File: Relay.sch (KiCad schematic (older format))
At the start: 0 parts

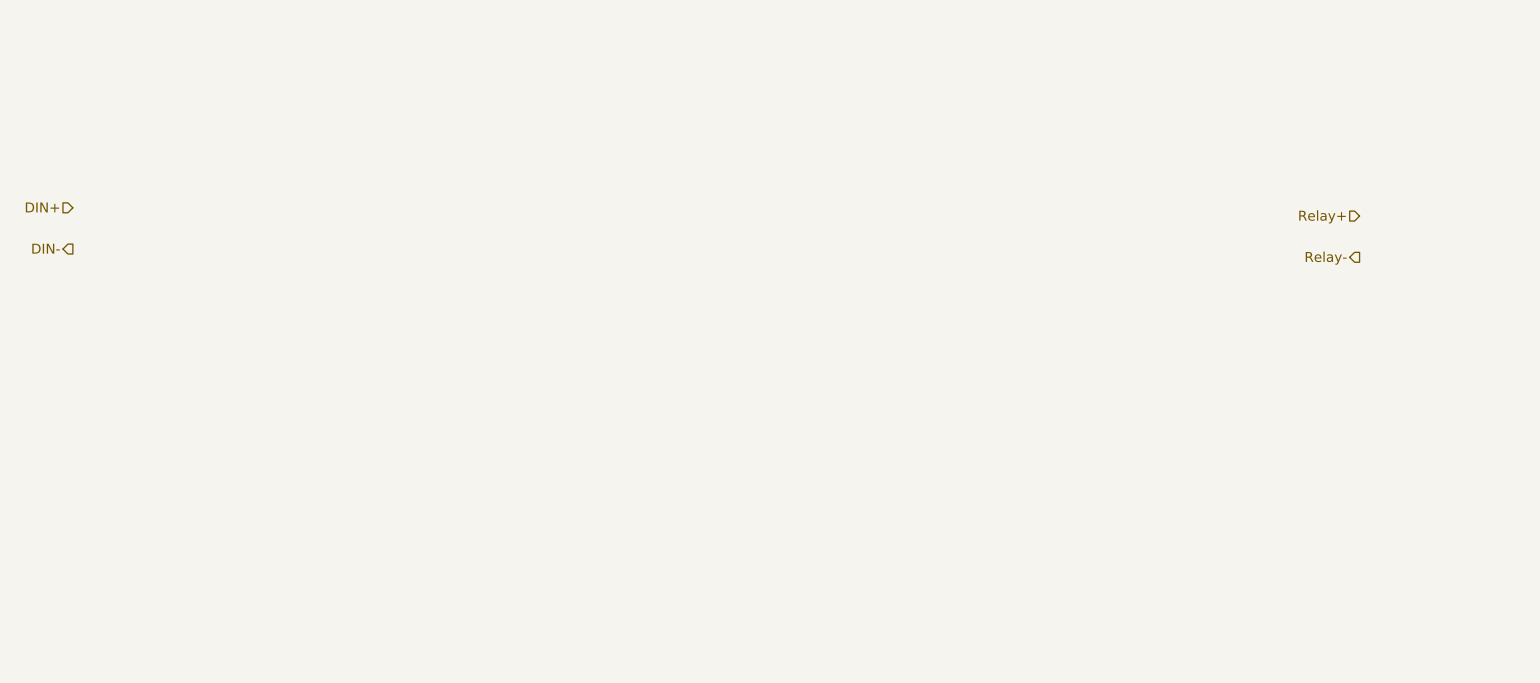
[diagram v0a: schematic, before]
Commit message: Module 3, Unit 5: Understanding The Relay Module
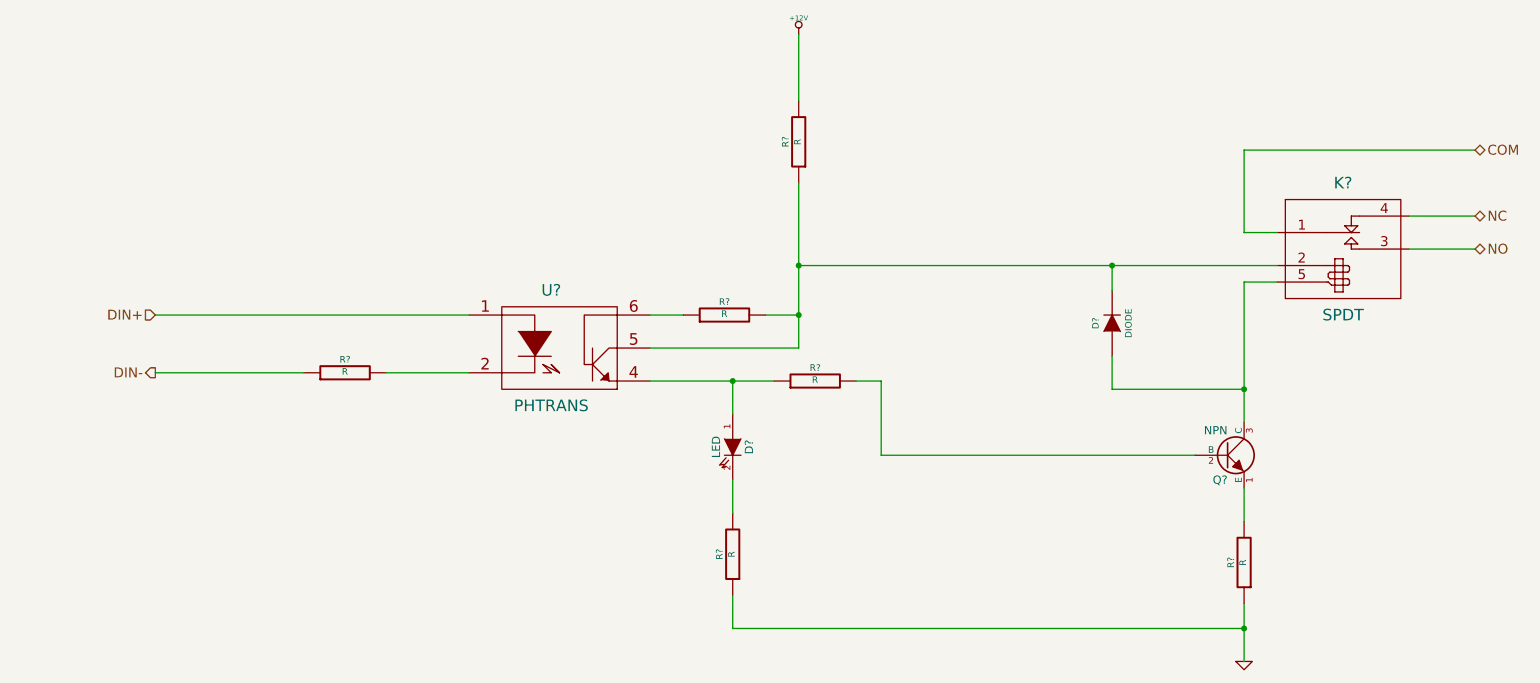
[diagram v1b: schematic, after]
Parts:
- added D?: LED, symbol LED
- added D?: DIODE, symbol DIODE
- added K?: SPDT, symbol SPDT
- added Q?: NPN, symbol NPN
- added R? (x6): R, symbol R
- added U?: PHTRANS, symbol PHTRANS
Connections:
- net DIN+: now also U?.1
- net DIN-: now also R?.1
- new net: R?.2, U?.2
- new net: D?.1 (A), R?.1, U?.4
- new net: D?.2 (K), K?.2 (COIL+), R?.1, R?.2, U?.5
- new net: R?.1, U?.6
- new net: Q?.2 (B), R?.2
- new net: Q?.1 (E), R?.2
- new net: D?.1 (A), K?.5 (COIL-), Q?.3 (C)
- new net: D?.2 (K), R?.2
- new net +12V: R?.2
- new net COM: K?.1 (COM)
- new net GND: R?.1, R?.1
- new net NC: K?.4 (NC)
- new net NO: K?.3 (NO)
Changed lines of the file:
@@
 LIBS:contrib
 LIBS:valves
+LIBS:BenchBudEE
 LIBS:BenchBudEE-cache
 EELAYER 24 0
@@
 Comment4 ""
 $EndDescr
-Text HLabel 2000 2550 0    60   Input ~ 0
+Text HLabel 2500 3200 0    60   Input ~ 0
 DIN+
-Text HLabel 2000 2800 0    60   Output ~ 0
+Text HLabel 2500 3550 0    60   Output ~ 0
 DIN-
-Text HLabel 9800 2600 0    60   Input ~ 0
-Relay+
-Text HLabel 9800 2850 0    60   Output ~ 0
-Relay-
+Text HLabel 10500 2600 2    60   BiDi ~ 0
+NC
+Text HLabel 10500 2800 2    60   BiDi ~ 0
+NO
+$Comp
+L PHTRANS U?
+U 1 1 53012FD3
+P 4950 3400
+F 0 "U?" H 4900 3750 70  0000 C CNN
+F 1 "PHTRANS" H 4900 3050 70  0000 C CNN
+F 2 "" H 4950 3400 60  0000 C CNN
+F 3 "" H 4950 3400 60  0000 C CNN
+	1    4950 3400
+	1    0    0    -1
+$EndComp
+$Comp
+L R R?
+U 1 1 53012FF1
+P 6500 3600
+F 0 "R?" V 6580 3600 40  0000 C CNN
+F 1 "R" V 6507 3601 40  0000 C CNN
+F 2 "" V 6430 3600 30  0000 C CNN
+F 3 "" H 6500 3600 30  0000 C CNN
+	1    6500 3600
+	0    -1   -1   0
+$EndComp
+$Comp
+L NPN Q?
+U 1 1 53013005
+P 9000 4050
+F 0 "Q?" H 9000 3900 50  0000 R CNN
+F 1 "NPN" H 9000 4200 50  0000 R CNN
+F 2 "" H 9000 4050 60  0000 C CNN
+F 3 "" H 9000 4050 60  0000 C CNN
+	1    9000 4050
+	1    0    0    -1
+$EndComp
+$Comp
+L LED D?
+U 1 1 53013023
+P 6000 4000
+F 0 "D?" H 6000 4100 50  0000 C CNN
+F 1 "LED" H 6000 3900 50  0000 C CNN
+F 2 "" H 6000 4000 60  0000 C CNN
+F 3 "" H 6000 4000 60  0000 C CNN
+	1    6000 4000
+	0    1    1    0
+$EndComp
+$Comp
+L SPDT K?
+U 1 1 5301353C
+P 9700 2650
+F 0 "K?" H 9700 2900 70  0000 C CNN
+F 1 "SPDT" H 9700 2100 70  0000 C CNN
+F 2 "" H 9700 2650 60  0000 C CNN
+F 3 "" H 9700 2650 60  0000 C CNN
+	1    9700 2650
+	1    0    0    -1
+$EndComp
+Text HLabel 10500 2200 2    60   BiDi ~ 0
+COM
+Wire Wire Line
+	10100 2600 10500 2600
+Wire Wire Line
+	10100 2800 10500 2800
+Wire Wire Line
+	5500 3600 6250 3600
+Wire Wire Line
+	9100 3000 9300 3000
+$Comp
+L GND #PWR?
+U 1 1 53013B82
+P 9100 5300
+F 0 "#PWR?" H 9100 5300 30  0001 C CNN
+F 1 "GND" H 9100 5230 30  0001 C CNN
+F 2 "" H 9100 5300 60  0000 C CNN
+F 3 "" H 9100 5300 60  0000 C CNN
+	1    9100 5300
+	1    0    0    -1
+$EndComp
+$Comp
+L R R?
+U 1 1 53013B9D
+P 9100 4700
+F 0 "R?" V 9180 4700 40  0000 C CNN
+F 1 "R" V 9107 4701 40  0000 C CNN
+F 2 "" V 9030 4700 30  0000 C CNN
+F 3 "" H 9100 4700 30  0000 C CNN
+	1    9100 4700
+	-1   0    0    1
+$EndComp
+Wire Wire Line
+	9100 4950 9100 5300
+$Comp
+L R R?
+U 1 1 53013BD9
+P 6000 4650
+F 0 "R?" V 6080 4650 40  0000 C CNN
+F 1 "R" V 6007 4651 40  0000 C CNN
+F 2 "" V 5930 4650 30  0000 C CNN
+F 3 "" H 6000 4650 30  0000 C CNN
+	1    6000 4650
+	-1   0    0    1
+$EndComp
+Wire Wire Line
+	6000 3800 6000 3600
+Connection ~ 6000 3600
+Wire Wire Line
+	6000 4200 6000 4400
+Wire Wire Line
+	6000 4900 6000 5100
+Wire Wire Line
+	6000 5100 9100 5100
+Connection ~ 9100 5100
+$Comp
+L R R?
+U 1 1 53013C23
+P 6400 2150
+F 0 "R?" V 6480 2150 40  0000 C CNN
+F 1 "R" V 6407 2151 40  0000 C CNN
+F 2 "" V 6330 2150 30  0000 C CNN
+F 3 "" H 6400 2150 30  0000 C CNN
+	1    6400 2150
+	-1   0    0    1
+$EndComp
+$Comp
+L +12V #PWR?
+U 1 1 53013C30
+P 6400 1500
+F 0 "#PWR?" H 6400 1450 20  0001 C CNN
+F 1 "+12V" H 6400 1600 30  0000 C CNN
+F 2 "" H 6400 1500 60  0000 C CNN
+F 3 "" H 6400 1500 60  0000 C CNN
+	1    6400 1500
+	1    0    0    -1
+$EndComp
+Wire Wire Line
+	6400 1500 6400 1900
+Wire Wire Line
+	6400 2400 6400 3400
+Wire Wire Line
+	6400 2900 9300 2900
+Wire Wire Line
+	6400 3400 5500 3400
+Connection ~ 6400 2900
+$Comp
+L R R?
+U 1 1 53013C87
+P 5950 3200
+F 0 "R?" V 6030 3200 40  0000 C CNN
+F 1 "R" V 5957 3201 40  0000 C CNN
+F 2 "" V 5880 3200 30  0000 C CNN
+F 3 "" H 5950 3200 30  0000 C CNN
+	1    5950 3200
+	0    -1   -1   0
+$EndComp
+Wire Wire Line
+	5500 3200 5700 3200
+Wire Wire Line
+	6200 3200 6400 3200
+Connection ~ 6400 3200
+$Comp
+L R R?
+U 1 1 53013CC0
+P 3650 3550
+F 0 "R?" V 3730 3550 40  0000 C CNN
+F 1 "R" V 3657 3551 40  0000 C CNN
+F 2 "" V 3580 3550 30  0000 C CNN
+F 3 "" H 3650 3550 30  0000 C CNN
+	1    3650 3550
+	0    -1   -1   0
+$EndComp
+Wire Wire Line
+	2500 3200 4400 3200
+Wire Wire Line
+	3900 3550 4400 3550
+Wire Wire Line
+	3400 3550 2500 3550
+Wire Wire Line
+	10500 2200 9100 2200
+Wire Wire Line
+	9100 2200 9100 2700
+Wire Wire Line
+	9100 2700 9300 2700
+$Comp
+L DIODE D?
+U 1 1 53013E0F
+P 8300 3250
+F 0 "D?" H 8300 3350 40  0000 C CNN
+F 1 "DIODE" H 8300 3150 40  0000 C CNN
+F 2 "" H 8300 3250 60  0000 C CNN
+F 3 "" H 8300 3250 60  0000 C CNN
+	1    8300 3250
+	0    -1   -1   0
+$EndComp
+Wire Wire Line
+	9100 3000 9100 3850
+Wire Wire Line
+	8300 2900 8300 3050
+Connection ~ 8300 2900
+Wire Wire Line
+	8300 3450 8300 3650
+Wire Wire Line
+	8300 3650 9100 3650
+Connection ~ 9100 3650
+Wire Wire Line
+	9100 4250 9100 4450
+Wire Wire Line
+	6750 3600 6900 3600
+Wire Wire Line
+	6900 3600 6900 4050
+Wire Wire Line
+	6900 4050 8800 4050
 $EndSCHEMATC
